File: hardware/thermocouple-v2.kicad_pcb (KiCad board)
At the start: 2 copper layers, 40 x 30 mm, 35 parts, among them J101 THERM, P1 CON-SENSOR2, P2 DEBUG, P3 BOOT, U1 XMC1100, U102 MAX31856, U103 DRILL, U104 DRILL, U105 DRILL, U106 DRILL

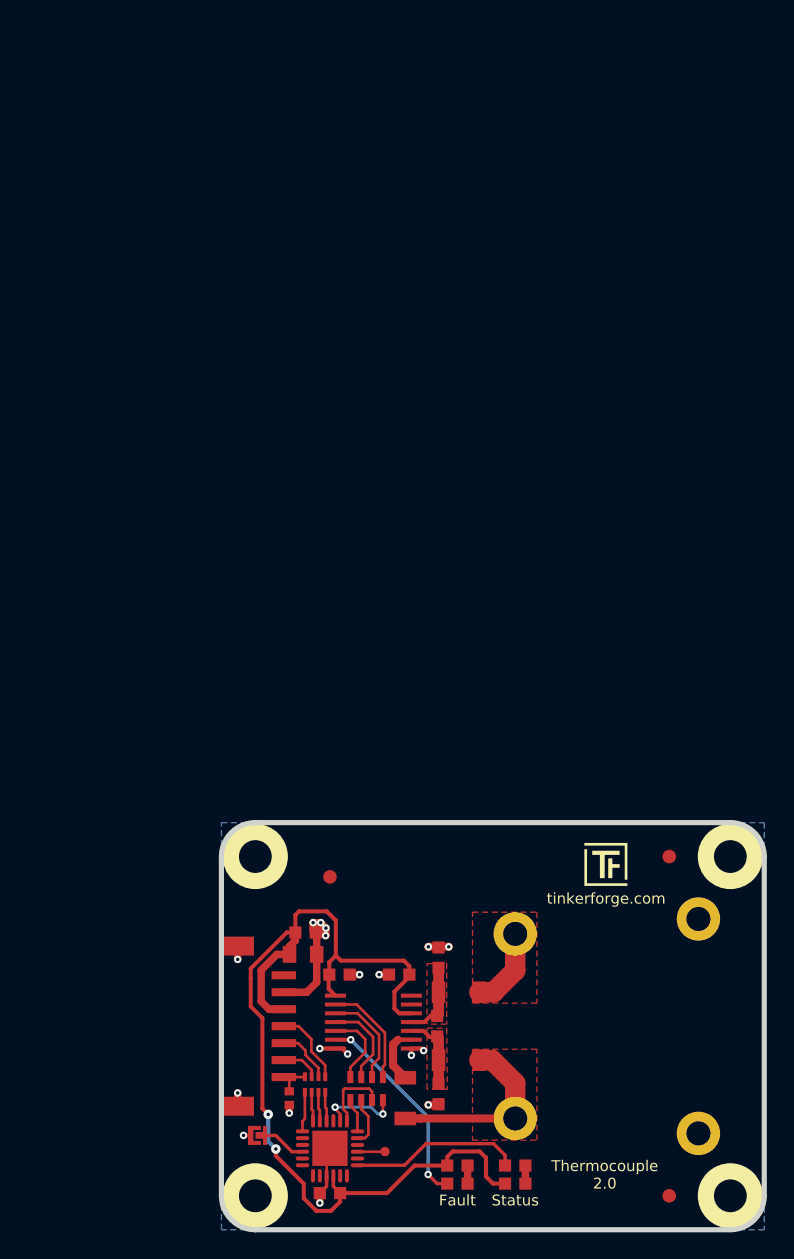
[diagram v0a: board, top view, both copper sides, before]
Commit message: Data Cleanup
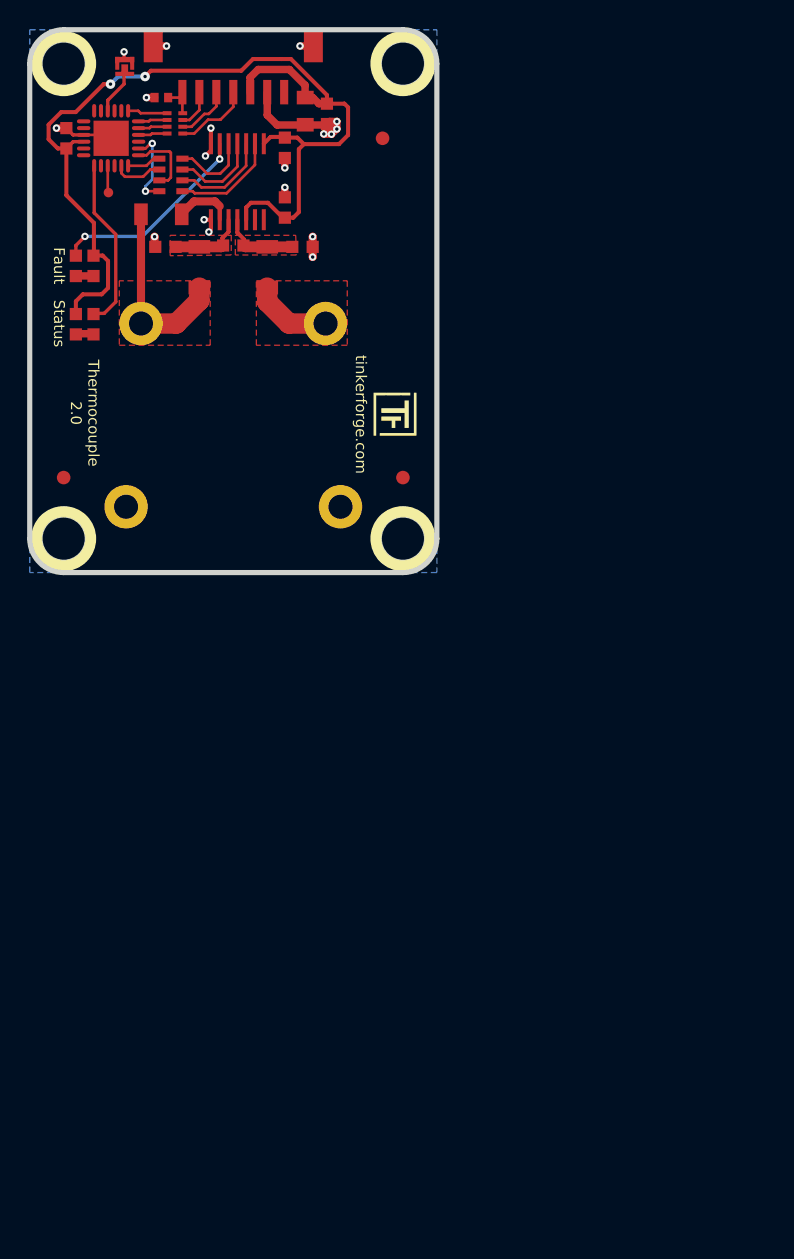
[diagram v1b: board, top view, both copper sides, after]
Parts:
- moved U104 84.6 mm to (138.5, 69.0), turned to -90 degrees
- moved C4 80.1 mm to (138.7, 74.5), turned to 90 degrees
- moved P3 79.4 mm to (143.0, 69.2), turned to -90 degrees
- moved U1 76.2 mm to (142.0, 74.5), turned to -90 degrees
- moved C1 74.3 mm to (145.7, 71.5), turned to 180 degrees
- moved P2 73.5 mm to (141.8, 78.5), turned to -90 degrees
- moved P1 73.4 mm to (151.0, 66.5), turned to 180 degrees
- moved D101 73.2 mm to (139.4, 83.9), turned to 90 degrees
- moved RP1 71.6 mm to (146.7, 73.4), turned to 90 degrees
- moved R101 71.5 mm to (140.7, 83.9), turned to 90 degrees
- moved D1 71.1 mm to (139.4, 88.2), turned to -90 degrees
- moved R1 69.3 mm to (140.7, 88.2), turned to -90 degrees
- moved Fiducial_Mark 69.2 mm to (138.5, 99.5), turned to -90 degrees
- moved U105 69.0 mm to (138.5, 104.0), turned to -90 degrees
- moved RP101 68.9 mm to (146.4, 77.2), turned to -90 degrees
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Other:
- board size 40 x 30 mm -> 30 x 40 mm
- net class Default removed
- board text added: "Copyright Tinkerforge GmbH 2023. This documentation describes Open Hardware and is licensed under the CERN OHL v. 1.1. You may redistribute and modify this documentation under the terms of the CERN OHL v.1.1. (http://ohwr.org/cernohl). This documentation is distributed WITHOUT ANY EXPRESS OR IMPLIED WARRANTY, INCLUDING OF MERCHANTABILITY, SATISFACTORY QUALITY AND FITNESS FOR A PARTICULAR PURPOSE.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"
- board text removed: "Copyright Tinkerforge GmbH 2018. This documentation describes Open Hardware and is licensed under the CERN OHL v. 1.1. You may redistribute and modify this documentation under the terms of the CERN OHL v.1.1. (http://ohwr.org/cernohl). This documentation is distributed WITHOUT ANY EXPRESS OR IMPLIED WARRANTY, INCLUDING OF MERCHANTABILITY, SATISFACTORY QUALITY AND FITNESS FOR A PARTICULAR PURPOSE.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"
